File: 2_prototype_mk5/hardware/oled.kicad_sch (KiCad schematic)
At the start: 1 part, among them J6 Conn_01x04_Pin

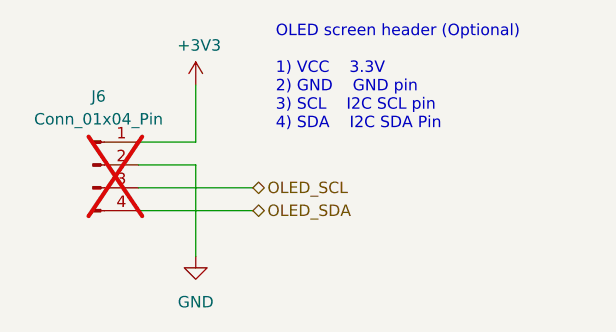
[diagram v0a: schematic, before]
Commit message: MK5 revision 2 hardware updates and ISA adapter revisions
Ignore VSCode local-history artifacts going forward.

Co-Authored-By: Claude Sonnet 5 <noreply@anthropic.com>
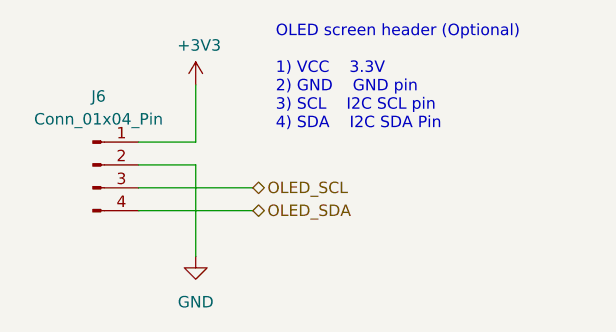
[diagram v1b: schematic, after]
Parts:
- J6: now fitted; now in the parts list
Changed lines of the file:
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@@
 		(body_style 1)
 		(exclude_from_sim no)
-		(in_bom no)
+		(in_bom yes)
 		(on_board yes)
 		(in_pos_files yes)
-		(dnp yes)
+		(dnp no)
 		(fields_autoplaced yes)
 		(property "Reference" "J6"
